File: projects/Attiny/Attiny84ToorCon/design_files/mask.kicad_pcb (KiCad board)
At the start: 2 copper layers, 63.5 x 101.6 mm, 44 parts, among them CON1 AVR-ISP-6, P0 CONN_01X01, P1 CONN_01X01, P2 CONN_01X01, P3 CONN_01X01, P4 CONN_01X01, P5 CONN_01X01, P6 CONN_01X01, P7 CONN_01X01, P8 CONN_01X01, P9 CONN_01X01, SW1 SW_SPDT, SW2 Fingerprint, U1 ATTINY84A-SSU, X1 Badgelife_shitty_connector

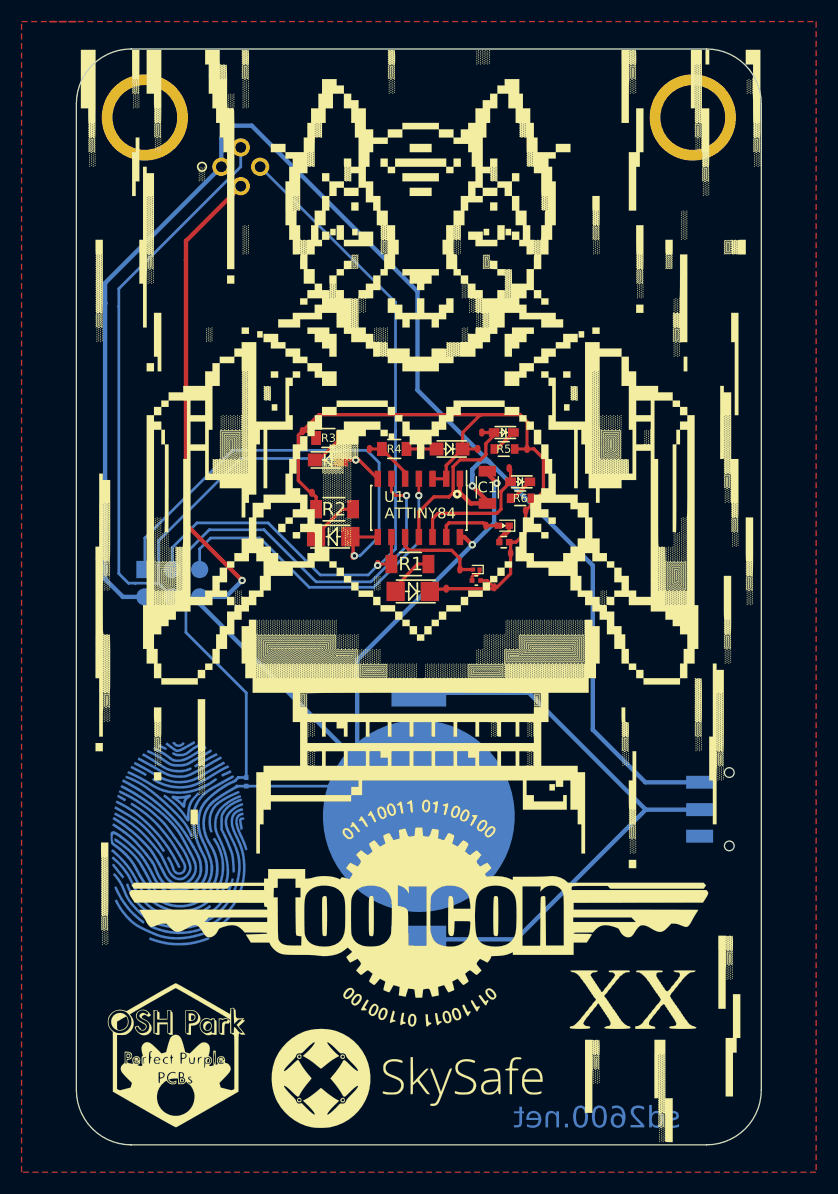
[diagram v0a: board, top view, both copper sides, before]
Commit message: Updates
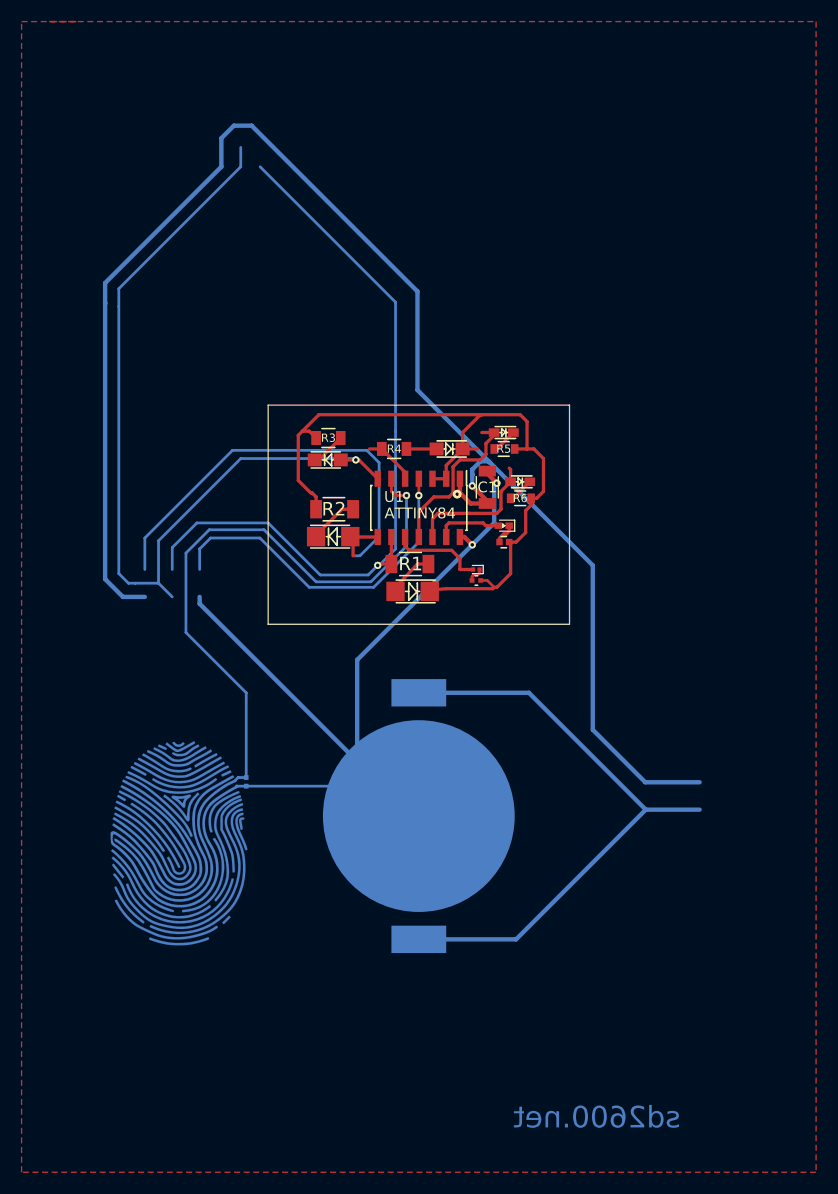
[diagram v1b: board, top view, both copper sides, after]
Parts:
- removed CON1: AVR-ISP-6, footprints:AVR-ISP-6
- removed the G*** at (123.2, 123.2)
- removed P0, P1: CONN_01X01, footprints:Pin_Header_Straight_1x01
- removed P2, P3, P4, P5, P6, P7, P8, P9, PG1, PG2, PG3, PG4, PG5, PG6, PG7, PG8: CONN_01X01, footprints:testPad
- removed SW1: SW_SPDT, footprints:SPST_SMD
- removed X1: Badgelife_shitty_connector, footprints:Badgelife-Shitty-2x2
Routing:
- net GND: track 134.1 -> 88.7 mm, vias 3 -> 2
- net /MISO: track 42.9 -> 4.56 mm, vias 1 -> 0
- net (no net): track 0.00 -> 38.4 mm
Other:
- board size 63.5 x 101.6 mm -> 27.9 x 20.3 mm
